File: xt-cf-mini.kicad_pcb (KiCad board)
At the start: 2 copper layers, 81.3 x 49 mm, 32 parts, among them P1 CF_CARD, P2 LED, SW1 ROM Enable, SW2 ROM Write Enable, SW3 ROM Addr, SW4 IDE Addr, U1 28C64, U2 74LS688, U3 74LS688, U4 74LS32, U5 74LS04

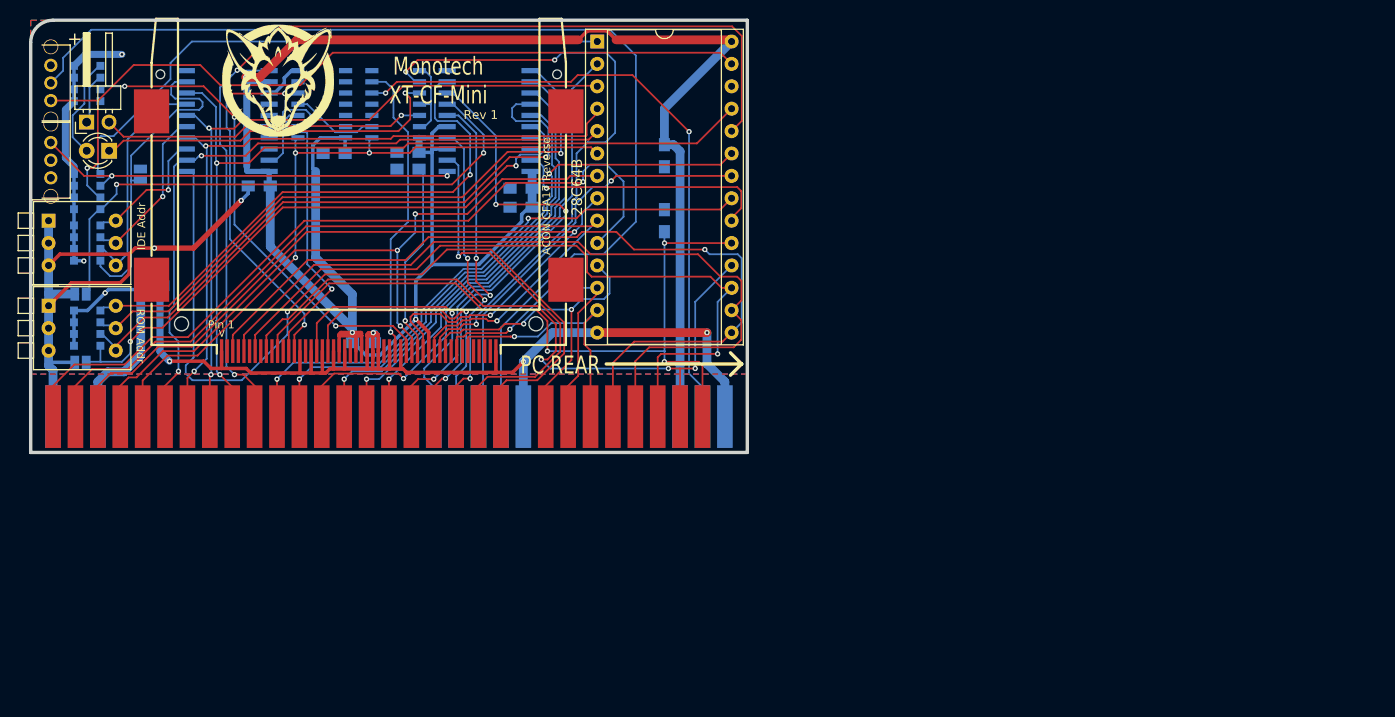
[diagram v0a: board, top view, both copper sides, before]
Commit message: Add files via upload
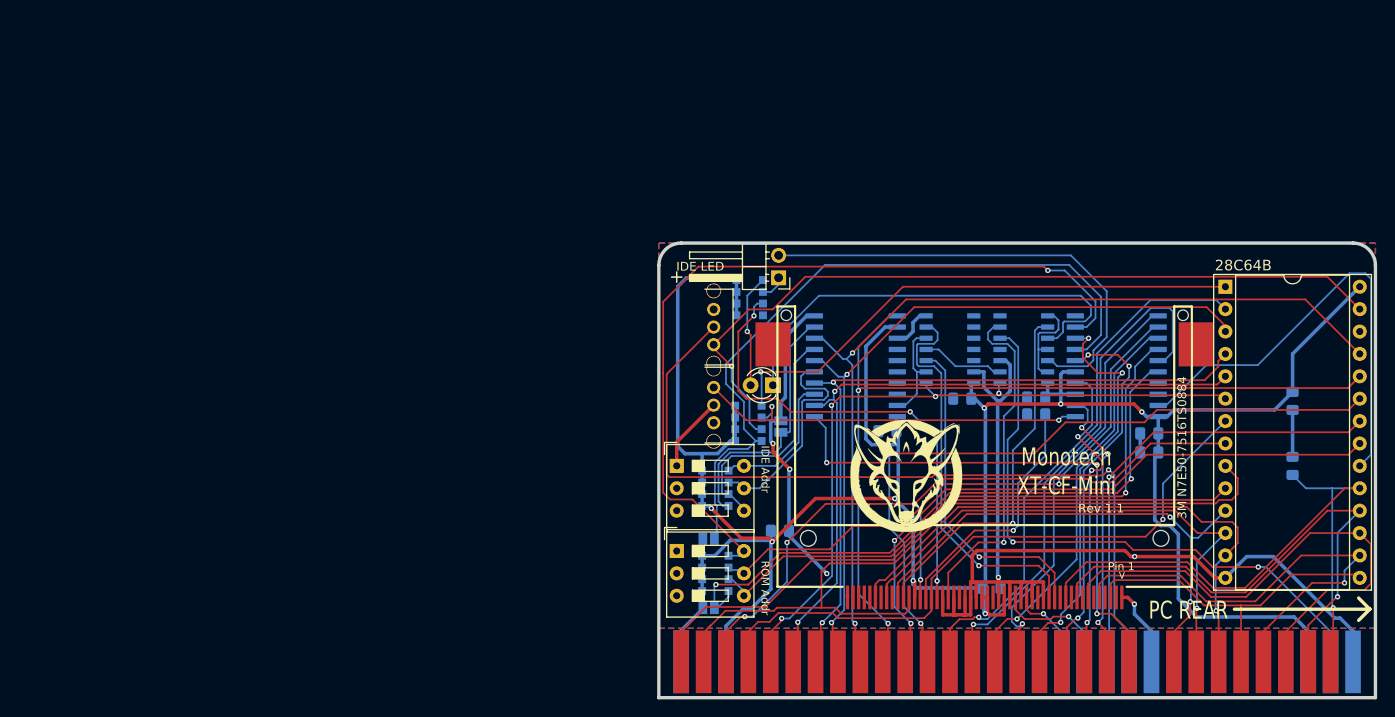
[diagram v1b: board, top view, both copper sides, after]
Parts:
- removed REF***: OSHW-Logo_7.5x8mm_SilkScreen, Symbols:OSHW-Logo_7.5x8mm_SilkScreen
- added G***: LOGO, Custom:Monotech_Logo_150, B.Cu at (215.5, 139.1)
- C1, C2, C3, C4, C5, C6: value 0.1uF -> 100nF; footprint Capacitors_SMD:C_0805_HandSoldering -> Capacitor_SMD:C_0805_2012Metric_Pad1.15x1.40mm_HandSolder
- C7, C8, R1, R2: footprint Capacitors_SMD:C_0805_HandSoldering -> Capacitor_SMD:C_0805_2012Metric_Pad1.15x1.40mm_HandSolder
- D1: value LED -> IDE LED; footprint LEDs:LED_D3.0mm -> LED_THT:LED_D3.0mm
- JP1, JP2, JP3: footprint Custom:SolderJumper-2_P1.3mm_Open_Pad1.0x1.5mm -> Jumper:SolderJumper-2_P1.3mm_Open_Pad1.0x1.5mm
- P1: footprint Custom:CF_Slot_ACON_CFA17_Reverse -> Custom:CF_Slot_3M_N7E50-7516TS0884
- P2: value LED -> IDE LED; footprint Pin_Headers:Pin_Header_Angled_1x02_Pitch2.54mm -> Connector_PinHeader_2.54mm:PinHeader_1x02_P2.54mm_Horizontal
- RN1, RN2, RN3, RN4: footprint Resistors_SMD:R_Array_Convex_4x1206 -> Resistor_SMD:R_Array_Convex_4x1206
- SW3, SW4: footprint Buttons_Switches_THT:SW_DIP_x3_W7.62mm_Piano -> Button_Switch_THT:SW_DIP_SPSTx03_Slide_9.78x9.8mm_W7.62mm_P2.54mm
- U1: footprint Housings_DIP:DIP-28_W15.24mm_Socket -> Package_DIP:DIP-28_W15.24mm_Socket
- U2, U3: footprint Housings_SOIC:SOIC-20W_7.5x12.8mm_Pitch1.27mm -> Package_SO:SOIC-20W_7.5x12.8mm_P1.27mm
- U4, U5: footprint Housings_SOIC:SOIC-14_3.9x8.7mm_Pitch1.27mm -> Package_SO:SOIC-14_3.9x8.7mm_P1.27mm
- moved G*** 84.2 mm to (200.9, 137.3)
- moved P2 80.4 mm to (186.4, 114.8), turned to 180 degrees
- moved SW1 80.2 mm to (179.1, 129.3)
- moved SW2 80.1 mm to (179.1, 120.4)
- moved D1 79.9 mm to (185.8, 127.0)
- moved RN2 79.5 mm to (183.0, 131.3)
- moved RN4 79.0 mm to (183.2, 117.1)
- moved JP3 78.1 mm to (186.7, 131.7)
- moved C2 76.5 mm to (228.5, 132.5)
- moved C4 76.5 mm to (207.3, 128.5)
- moved C8 76.5 mm to (228.5, 134.6)
- moved R2 76.5 mm to (244.7, 136.1)
- moved U1 76.5 mm to (237.1, 115.8)
- moved C1 76.5 mm to (244.7, 128.8)
- moved C5 76.5 mm to (198.8, 132.2)
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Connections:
- net /RESETDRV renamed /RSTDRV
- P1 pad 24: (no net) -> Net-(P1-Pad24)
- P1 pad 25: (no net) -> Net-(P1-Pad25)
- P1 pad 26: (no net) -> Net-(P1-Pad26)
- P1 pad 27: (no net) -> Net-(P1-Pad27)
- P1 pad 28: (no net) -> Net-(P1-Pad28)
- P1 pad 29: (no net) -> Net-(P1-Pad29)
- P1 pad 30: (no net) -> Net-(P1-Pad30)
- P1 pad 31: (no net) -> Net-(P1-Pad31)
- P1 pad 33: (no net) -> Net-(P1-Pad33)
- P1 pad 37: (no net) -> Net-(P1-Pad37)
- P1 pad 40: (no net) -> Net-(P1-Pad40)
- P1 pad 46: (no net) -> Net-(P1-Pad46)
- P1 pad 47: (no net) -> Net-(P1-Pad47)
- P1 pad 48: (no net) -> Net-(P1-Pad48)
- P1 pad 49: (no net) -> Net-(P1-Pad49)
- RN4 pad 4: (no net) -> Net-(RN4-Pad4)
- SW1 pad 3: (no net) -> Net-(SW1-Pad3)
- SW2 pad 1: (no net) -> Net-(SW2-Pad1)
- U1 pad 26: (no net) -> Net-(U1-Pad26)
- U4 pad 11: (no net) -> Net-(U4-Pad11)
- U4 pad 8: (no net) -> Net-(U4-Pad8)
- U5 pad 4: (no net) -> Net-(U5-Pad4)
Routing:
- net /D3: track 95.5 -> 39.2 mm, vias 1 -> 0
- net /D4: track 91.4 -> 53.6 mm, vias 0 -> 1
- net /D2: track 30.5 -> 63.6 mm
- net /AEN: track 94.1 -> 61.4 mm, vias 1 -> 3
- net Net-(RN3-Pad1): track 62.8 -> 92.4 mm
- net /~CF_DASP: track 70.9 -> 41.4 mm, vias 3 -> 1
- net /~MEMW: track 120.2 -> 92.3 mm, vias 0 -> 1
- net /D5: track 84.9 -> 58.7 mm, vias 1 -> 0
- net /D1: track 35.8 -> 60.4 mm
- net /~IOR: track 33.1 -> 9.82 mm
- net /D6: track 81.2 -> 59.1 mm, vias 3 -> 1
- net /~ROM_CS: track 30.5 -> 52.3 mm, vias 1 -> 0
- net /D0: track 39.5 -> 59.3 mm
- net /~IOW: track 32.4 -> 13.8 mm
- net Net-(JP1-Pad2): track 64.7 -> 82.0 mm, vias 2 -> 0
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- added copper zone on F.Cu, net GND
- removed copper zone on F.Cu, net VCC
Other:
- board size 81.3 x 49 mm -> 81.3 x 51.6 mm
- rule pad_to_mask_clearance: 0.254 -> 0
- board text added: "123 111 300 011 320 101 340 001 360 110 380 010 3A0 100 3C0 000 3E0"
- board text added: "Rev 1.1"
- board text removed: "123 111 300 110 320 101 340 100 360 011 380 010 3A0 001 3C0 000 3E0"
- board text removed: "Rev 1"
